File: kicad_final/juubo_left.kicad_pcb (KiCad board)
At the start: 2 copper layers, 145.6 x 125.5 mm, 50 parts

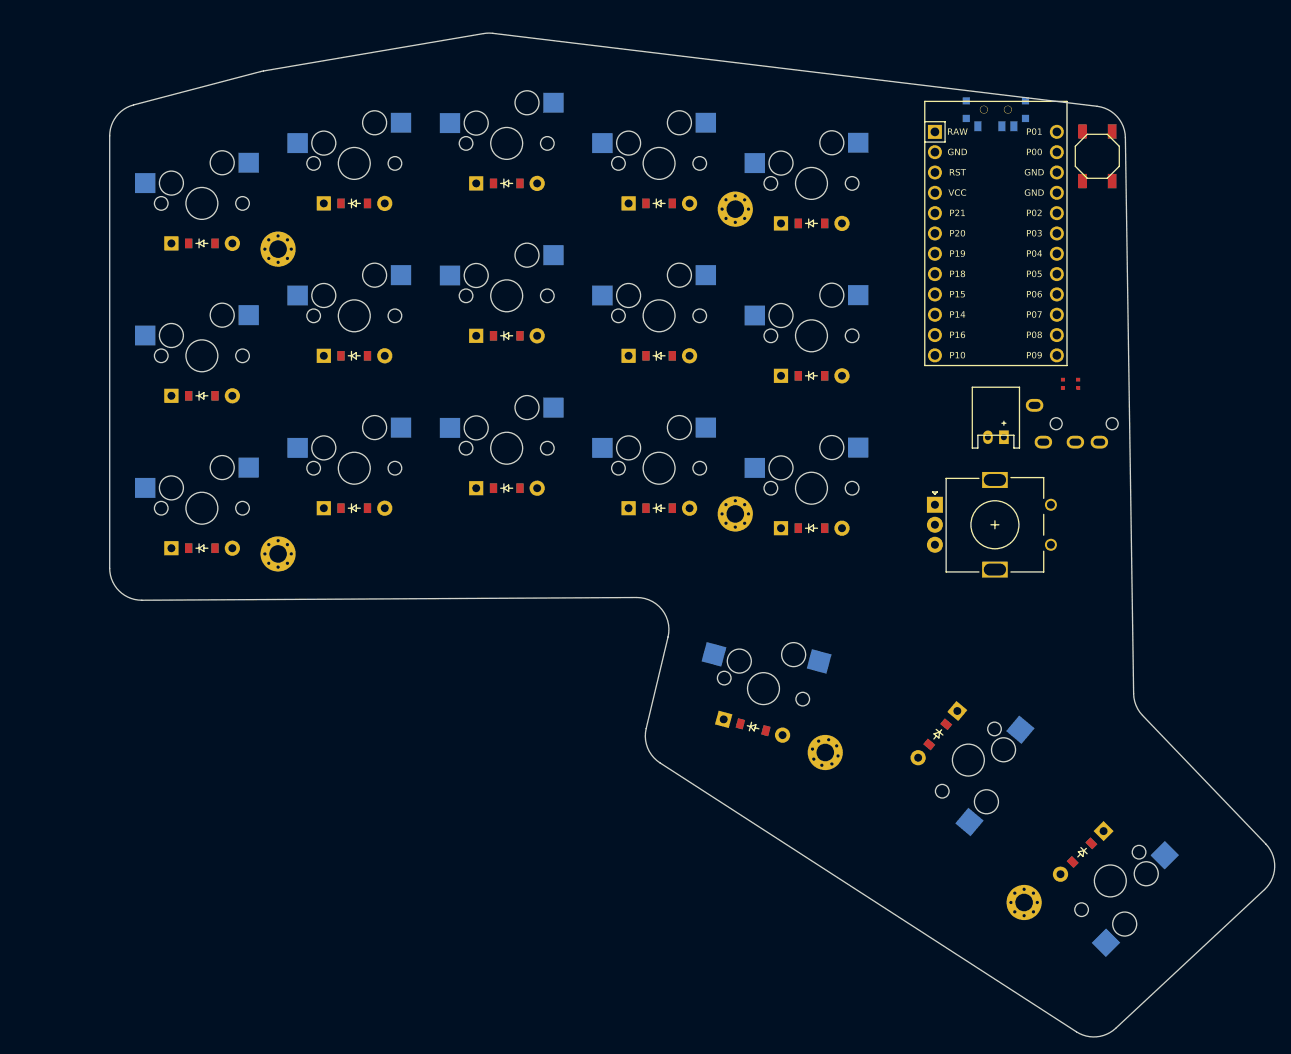
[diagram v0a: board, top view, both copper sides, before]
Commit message: Left routed
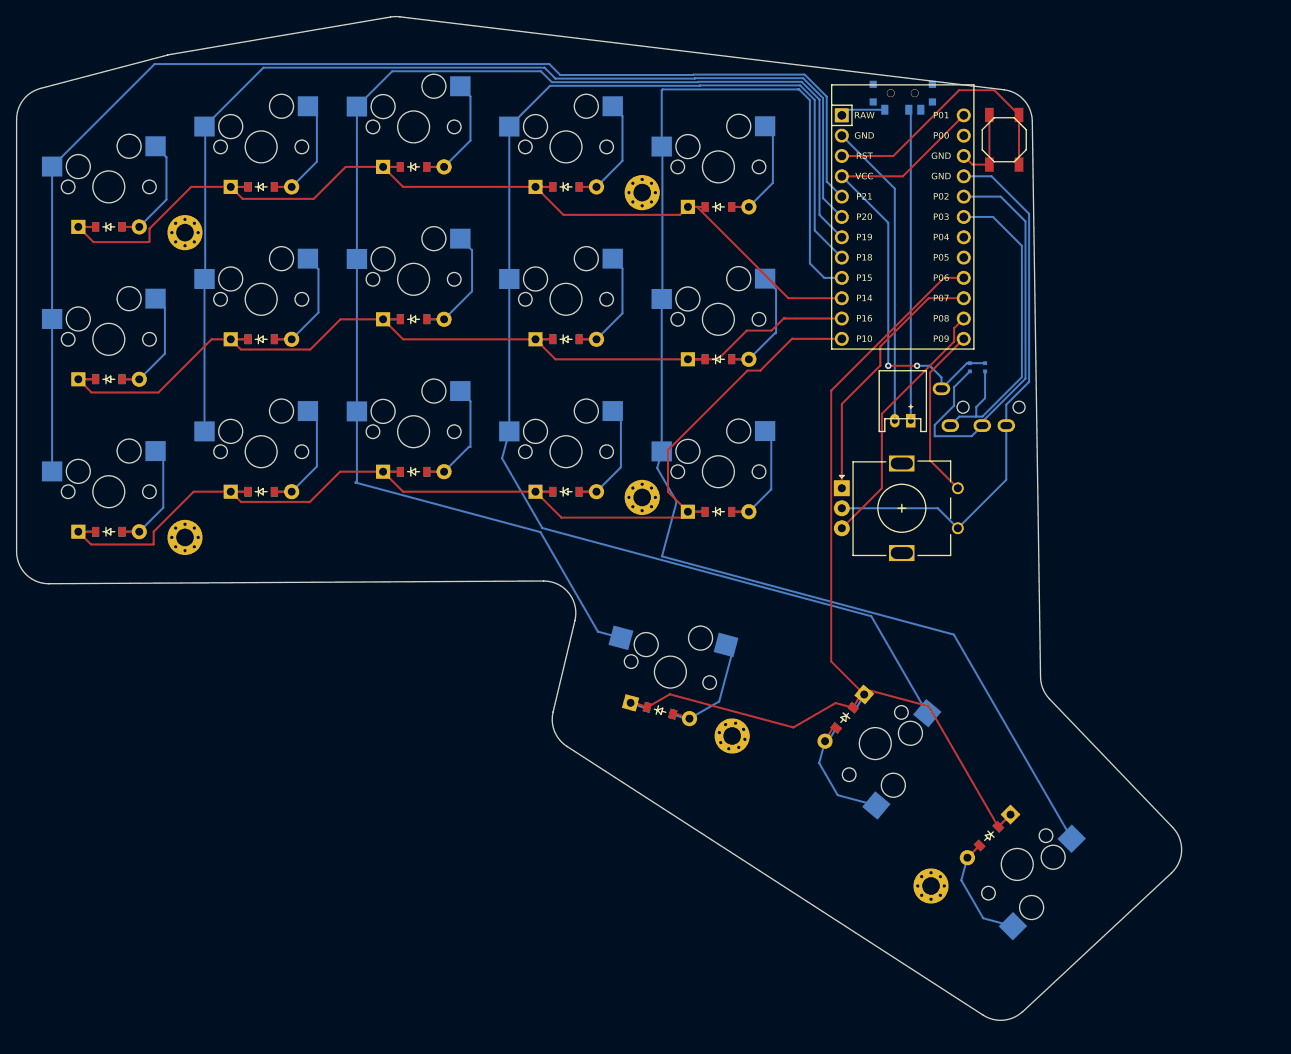
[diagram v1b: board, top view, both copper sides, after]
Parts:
- DISP1, DISP2: moved to B.Cu
- moved D5 11.8 mm to (107.4, 78.9)
- moved S9 11.8 mm to (126.5, 52.3)
- moved S14 11.8 mm to (164.6, 76.4)
- moved S17 11.8 mm to (184.2, 129.4)
- moved D11 11.8 mm to (145.5, 78.9)
- moved D9 11.8 mm to (126.5, 57.3)
- moved S5 11.8 mm to (107.4, 73.9)
- moved _6 11.8 mm to (155.0, 98.7)
- moved D1 11.8 mm to (88.4, 102.9)
- moved D8 11.8 mm to (126.5, 76.4)
- moved S7 11.8 mm to (126.5, 90.4)
- moved D6 11.8 mm to (107.4, 59.8)
- moved S2 11.8 mm to (88.4, 78.9)
- moved D10 11.8 mm to (145.5, 97.9)
- moved S18 11.8 mm to (201.9, 144.5)
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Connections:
- MCU1 pad 13: P1 -> VCC
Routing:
- net P15: track 0.00 -> 170.8 mm
- net P18: track 0.00 -> 170.4 mm
- net P19: track 0.00 -> 167.9 mm
- net P21: track 0.00 -> 155.2 mm
- net P10: track 0.00 -> 143.2 mm
- net P20: track 0.00 -> 136.0 mm
- net P14: track 0.00 -> 131.5 mm
- net P6: track 0.00 -> 128.9 mm
- net P16: track 0.00 -> 126.8 mm
- net GND: track 0.00 -> 116.9 mm
- net VCC: track 0.00 -> 60.1 mm, vias 0 -> 2
- net P2: track 0.00 -> 53.7 mm
- net P3: track 0.00 -> 43.1 mm
- net B+: track 0.00 -> 39.0 mm
- net RST: track 0.00 -> 33.0 mm
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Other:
- outline, holes or cut-outs redrawn
- net class Default removed
